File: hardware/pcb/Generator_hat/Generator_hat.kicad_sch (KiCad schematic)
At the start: 18 parts, among them J1 Screw_Terminal_01x03, J2 Screw_Terminal_01x02, U1 DHT11

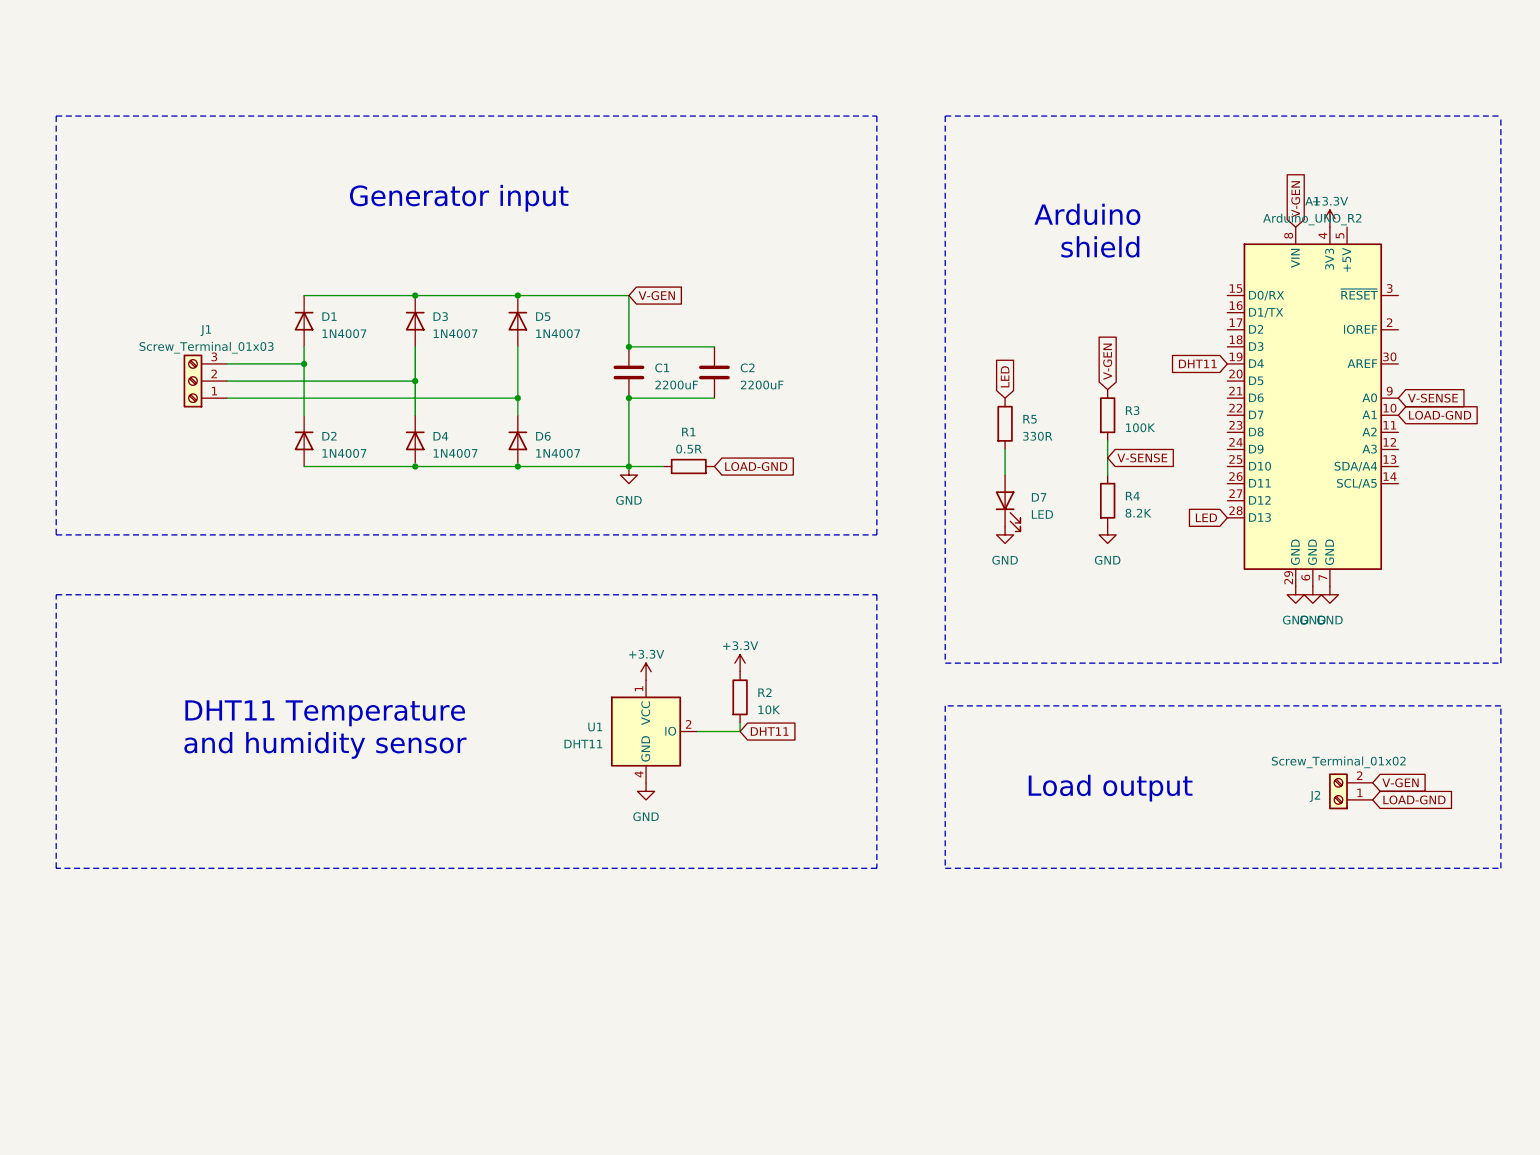
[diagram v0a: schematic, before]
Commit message: update pcb
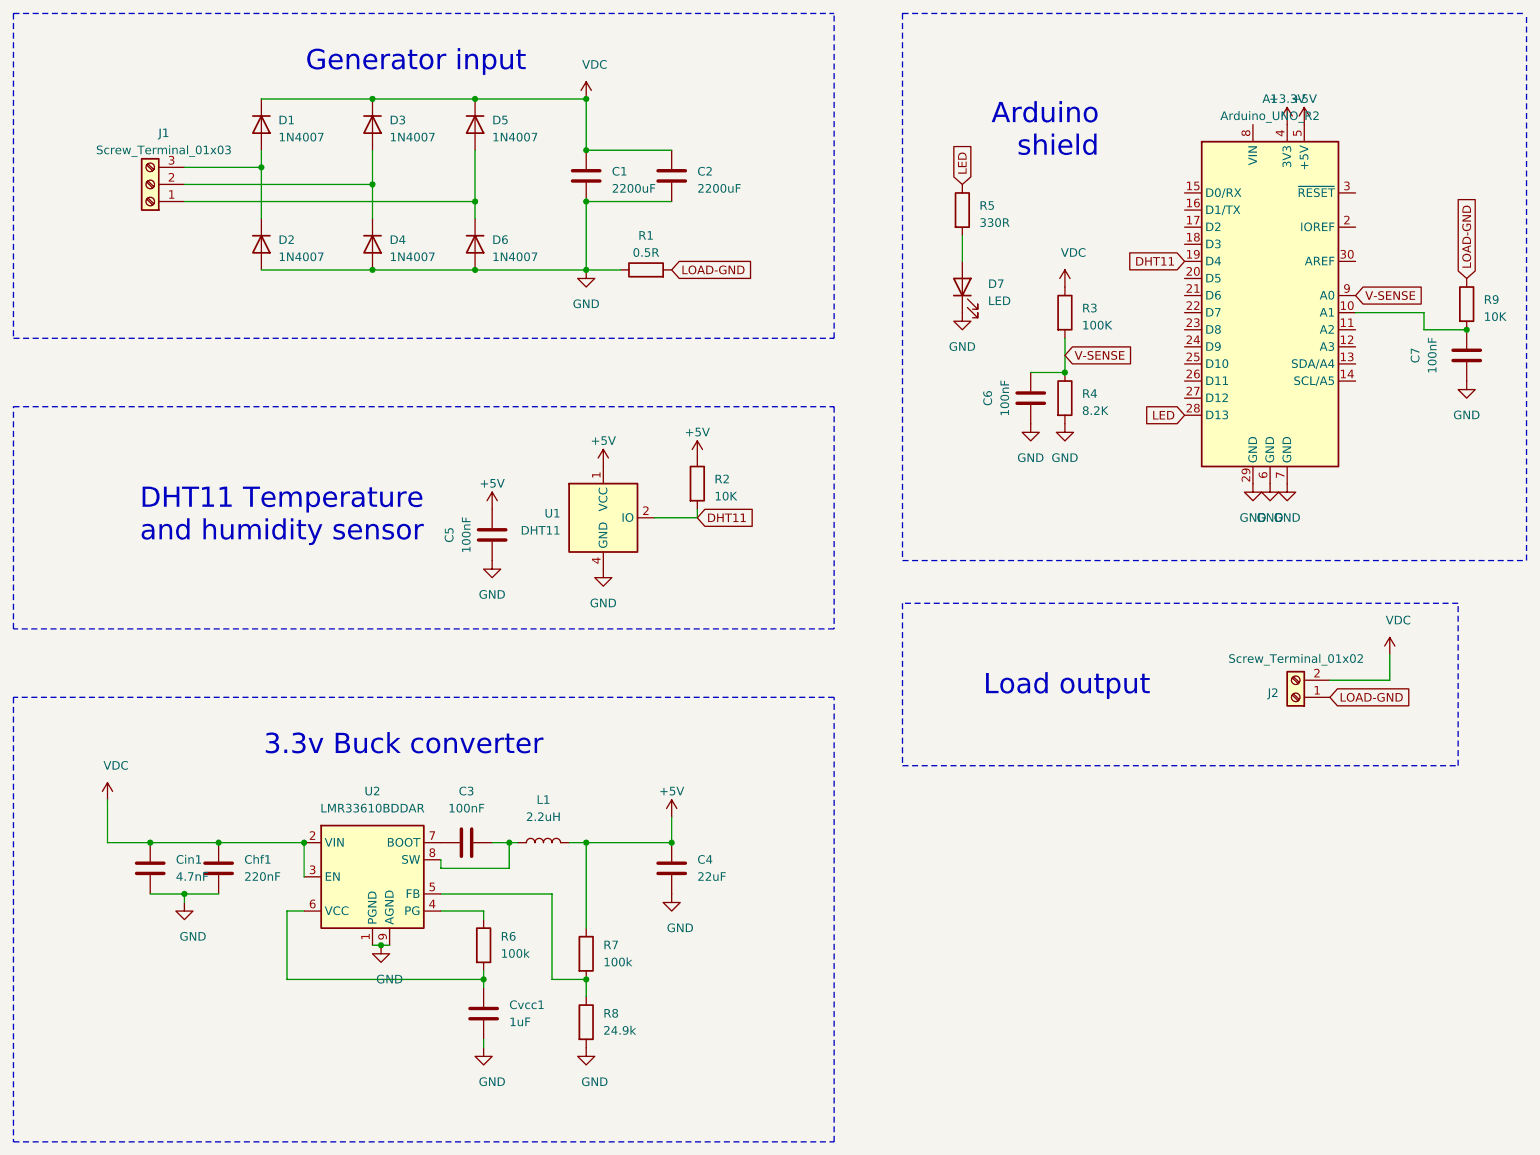
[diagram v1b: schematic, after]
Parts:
- added C3, C5, C6, C7: 100nF, Capacitor_SMD:C_0805_2012Metric_Pad1.18x1.45mm_HandSolder, symbol Device:C
- added C4: 22uF, Capacitor_SMD:CP_Elec_8x6.9, symbol Device:C
- added Chf1: 220nF, Capacitor_SMD:C_0805_2012Metric_Pad1.18x1.45mm_HandSolder, symbol Device:C
- added Cin1: 4.7nF, Capacitor_SMD:C_0805_2012Metric_Pad1.18x1.45mm_HandSolder, symbol Device:C
- added Cvcc1: 1uF, Capacitor_SMD:C_0805_2012Metric_Pad1.18x1.45mm_HandSolder, symbol Device:C
- added L1: 2.2uH, Inductor_SMD:L_Taiyo-Yuden_NR-50xx_HandSoldering, symbol Device:L
- added R6, R7: 100k, Resistor_SMD:R_0805_2012Metric_Pad1.20x1.40mm_HandSolder, symbol Device:R
- added R8: 24.9k, Resistor_SMD:R_0805_2012Metric_Pad1.20x1.40mm_HandSolder, symbol Device:R
- added R9: 10K, Resistor_SMD:R_0805_2012Metric_Pad1.20x1.40mm_HandSolder, symbol Device:R
- added U2: LMR33610BDDAR, Package_SO:Texas_HSOP-8-1EP_3.9x4.9mm_P1.27mm_ThermalVias, symbol Regulator_Switching:LMR33610BDDAR
- D1, D2, D3, D4, D5, D6: footprint Diode_THT:D_DO-41_SOD81_P10.16mm_Horizontal -> Diode_SMD:D_SMA
- R2, R3, R4, R5: footprint Resistor_THT:R_Axial_DIN0207_L6.3mm_D2.5mm_P10.16mm_Horizontal -> Resistor_SMD:R_0805_2012Metric_Pad1.20x1.40mm_HandSolder
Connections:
- net +3V3: no longer R2.1, U1.1 (VCC)
- net GND: now also C4.2, C5.2, C6.2, C7.2, Chf1.2, Cin1.2, Cvcc1.2, R8.2, U2.1 (PGND), U2.9 (AGND)
- net LOAD-GND: now also R9.1; no longer A1.10 (A1)
- net V-SENSE: now also C6.1
- net +5V: now reaches A1.5 (+5V)
- net +5V: now also R2.1, U1.1 (VCC), C4.1, C5.1, L1.2, R7.1
- net V-GEN renamed VDC
- net VDC: now also Chf1.1, Cin1.1, U2.2 (VIN), U2.3 (EN); no longer A1.8 (VIN)
- new net: Cvcc1.1, R6.2, U2.6 (VCC)
- new net: C3.1, L1.1, U2.8 (SW)
- new net: C3.2, U2.7 (BOOT)
- new net: R7.2, R8.1, U2.5 (FB)
- new net: A1.10 (A1), C7.1, R9.2
- new net: R6.1, U2.4 (PG)
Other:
- note added: "3.3v Buck converter"
- moved on the sheet: A1, C1, C2, D1, D2, D3, D4, D5, D6, D7, J1, J2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
